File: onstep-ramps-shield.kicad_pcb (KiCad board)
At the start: 2 copper layers, 120.7 x 67.3 mm, 25 parts

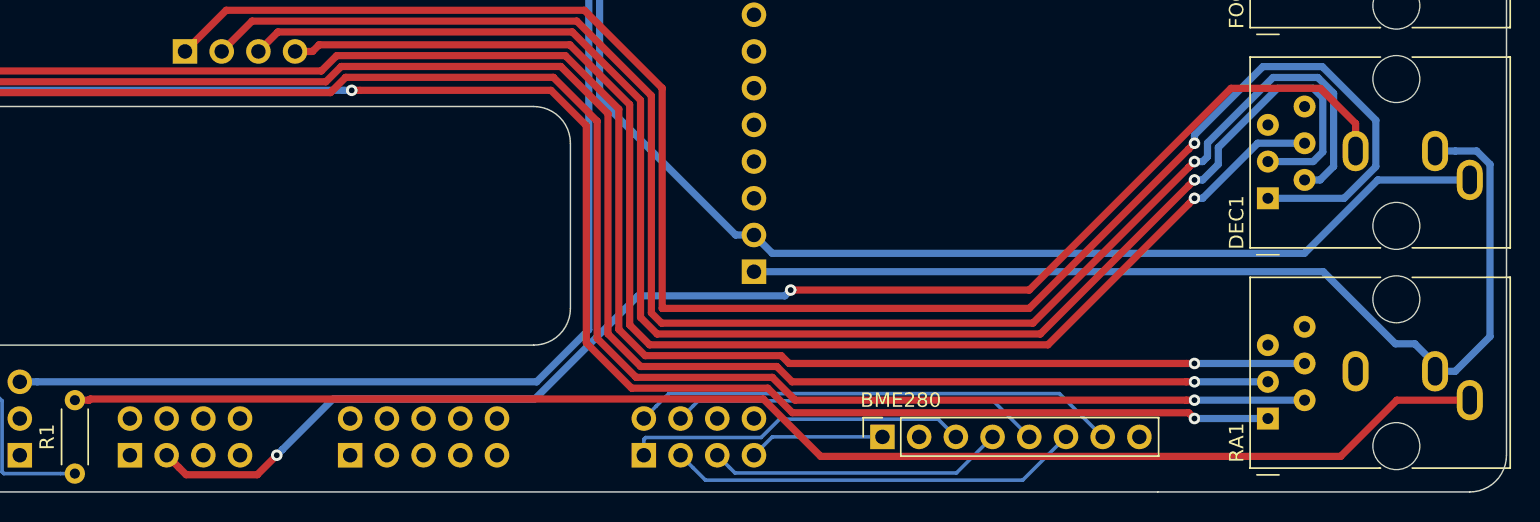
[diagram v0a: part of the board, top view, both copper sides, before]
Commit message: Routing
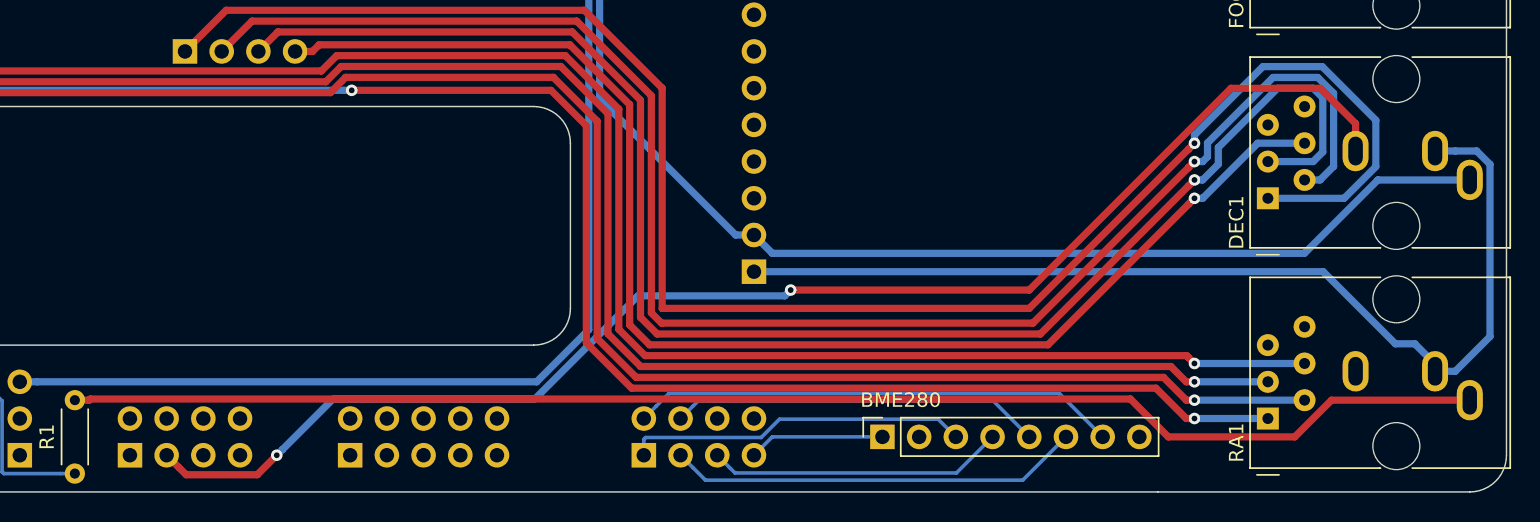
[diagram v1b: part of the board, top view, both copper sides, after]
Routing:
- net Net-(J_RET1-PadS): track 99.8 -> 98.7 mm
